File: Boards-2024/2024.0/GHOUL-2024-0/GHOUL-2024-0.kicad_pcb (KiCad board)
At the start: 4 copper layers, 57 x 60 mm, 106 parts, among them J1 USB_C_Receptacle_USB2.0, J2 U.FL, J3 SOICbite, J4 Conn_01x03_Pin, Q1 Q_NMOS_GSD, Q2 Q_NMOS_GSD, Q3 Q_NMOS_GSD, Q4 Q_NMOS_GSD, Q5 Q_NMOS_GSD, SW2 SLIDE, U1 MCU_RaspberryPi_RP2040_RP2040, U10 LTM4622AEV-PBF, U11 MAX-M10S, U2 TVS1800DRVR, U3 USBLC6-2SC6, U4 TPS2121RUXR, U5 W25Q128JVS, U6 LT6703CDC-3, U7 DRF1262TL, U8 MB85RS1MT, U9 MS5607-02BA, Y1 12MHz

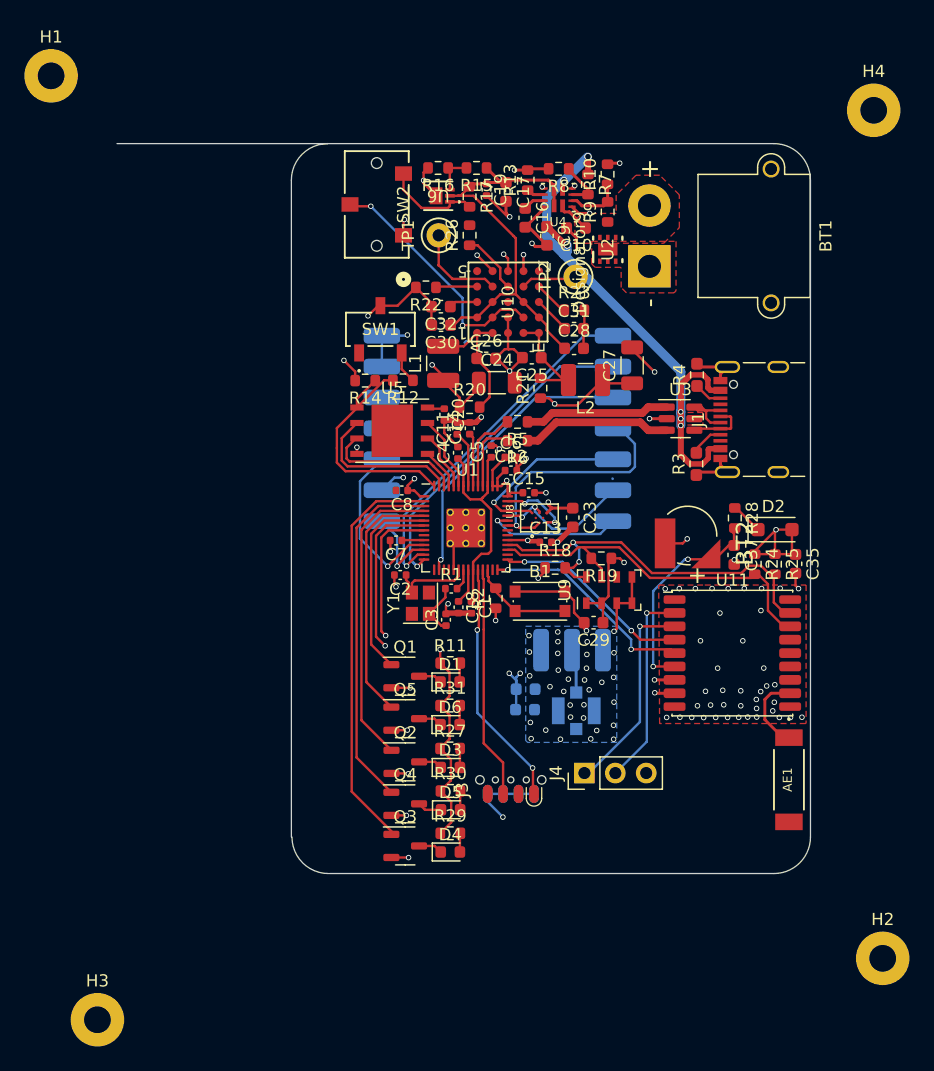
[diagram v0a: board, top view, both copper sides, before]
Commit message: finished board
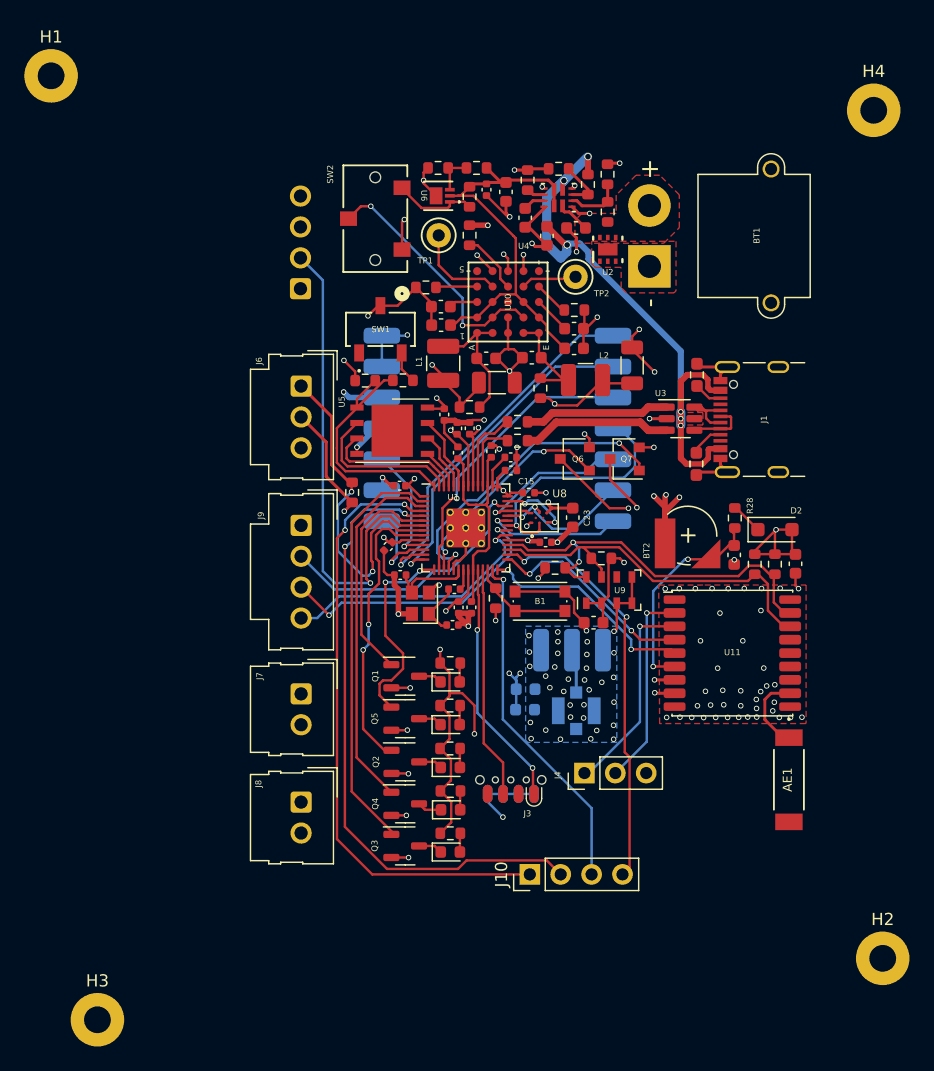
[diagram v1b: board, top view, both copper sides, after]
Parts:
- added J10: Conn_01x04, Connector_PinHeader_2.54mm:PinHeader_1x04_P2.54mm_Vertical, F.Cu at (156.9, 147.1)
- added J5: Conn_01x04, Connector_Molex:Molex_SL_171971-0004_1x04_P2.54mm_Vertical, B.Cu at (138.1, 98.9)
- added J6: Conn_01x03, Connector_Molex:Molex_SL_171971-0003_1x03_P2.54mm_Vertical, F.Cu at (138.1, 106.9)
- added J7: Conn_01x02, Connector_Molex:Molex_SL_171971-0002_1x02_P2.54mm_Vertical, F.Cu at (138.1, 132.2)
- added J8: Conn_01x02, Connector_Molex:Molex_SL_171971-0002_1x02_P2.54mm_Vertical, F.Cu at (138.1, 141.1)
- added J9: Conn_01x04, Connector_Molex:Molex_SL_171971-0004_1x04_P2.54mm_Vertical, F.Cu at (138.1, 118.4)
- added Q6: Q_NMOS_GSD, Package_TO_SOT_SMD:SC-59, F.Cu at (160.6, 112.9)
- added Q7: Q_NMOS_GSD, Package_TO_SOT_SMD:SC-59, F.Cu at (164.7, 112.9)
- added R32: 4.7k, Resistor_SMD:R_0603_1608Metric, F.Cu at (142.3, 115.7)
- moved SW2 1.18 mm to (144.2, 93.2)
- moved C7 0.81 mm to (145.3, 120.1), turned to -135 degrees
- moved C3 0.69 mm to (150.6, 126.6), turned to 0 degrees
- moved C8 0.43 mm to (146.2, 115.1)
- moved R1 0.26 mm to (150.7, 123.6)
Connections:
- U1 pad 15: unconnected-(U1-GPIO12-Pad15) -> /LED4
- U1 pad 17: unconnected-(U1-GPIO14-Pad17) -> /HEATER1
- U1 pad 18: unconnected-(U1-GPIO15-Pad18) -> /HEATER2
- U1 pad 27: unconnected-(U1-GPIO16-Pad27) -> /GPIO16
- U1 pad 30: unconnected-(U1-GPIO19-Pad30) -> /GPIO19
- U1 pad 34: unconnected-(U1-GPIO22-Pad34) -> /PGOOD_CUT
- U1 pad 35: unconnected-(U1-GPIO23-Pad35) -> /DATA_CUT
- U1 pad 4: /LED3 -> /GPIO2
- U1 pad 40: unconnected-(U1-GPIO28_ADC2-Pad40) -> /CUT_CURR
- U1 pad 5: /LED4 -> /GPIO3
- U1 pad 7: unconnected-(U1-GPIO5-Pad7) -> /SERVO_PWM
- U1 pad 8: unconnected-(U1-GPIO6-Pad8) -> /TEMP
- U1 pad 9: unconnected-(U1-GPIO7-Pad9) -> /LED3
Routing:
- net /GPIO3: track 0.00 -> 51.9 mm, vias 0 -> 2
- net /GPIO2: track 0.00 -> 50.8 mm, vias 0 -> 2
- net Net-(J8-Pin_2): track 0.00 -> 50.5 mm, vias 0 -> 1
- net Net-(J7-Pin_2): track 0.00 -> 45.1 mm, vias 0 -> 1
- net +5V: track 43.7 -> 87.0 mm
- net /SERVO_PWM: track 0.00 -> 40.8 mm, vias 0 -> 1
- net /GPIO19: track 0.00 -> 33.9 mm, vias 0 -> 2
- net GND: track 116.5 -> 149.2 mm, vias 109 -> 119
- net /GPIO16: track 0.00 -> 28.8 mm, vias 0 -> 1
- net /TEMP: track 0.00 -> 28.0 mm, vias 0 -> 2
- net /HEATER2: track 0.00 -> 26.3 mm, vias 0 -> 2
- net /DATA_CUT: track 0.00 -> 23.7 mm, vias 0 -> 2
- net /CUT_CURR: track 0.00 -> 22.6 mm, vias 0 -> 1
- net /PGOOD_CUT: track 0.00 -> 21.7 mm, vias 0 -> 1
- net +3V3: track 86.8 -> 106.5 mm, vias 13 -> 20
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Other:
- board outline removed
